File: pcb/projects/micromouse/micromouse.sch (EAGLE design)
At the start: 52 parts, among them M1 332-06, M2 332-06, U1 DSPIC33FJ64MC804-H/PT, U2 UA78M33CKCS, U3 UA78M05CKCS

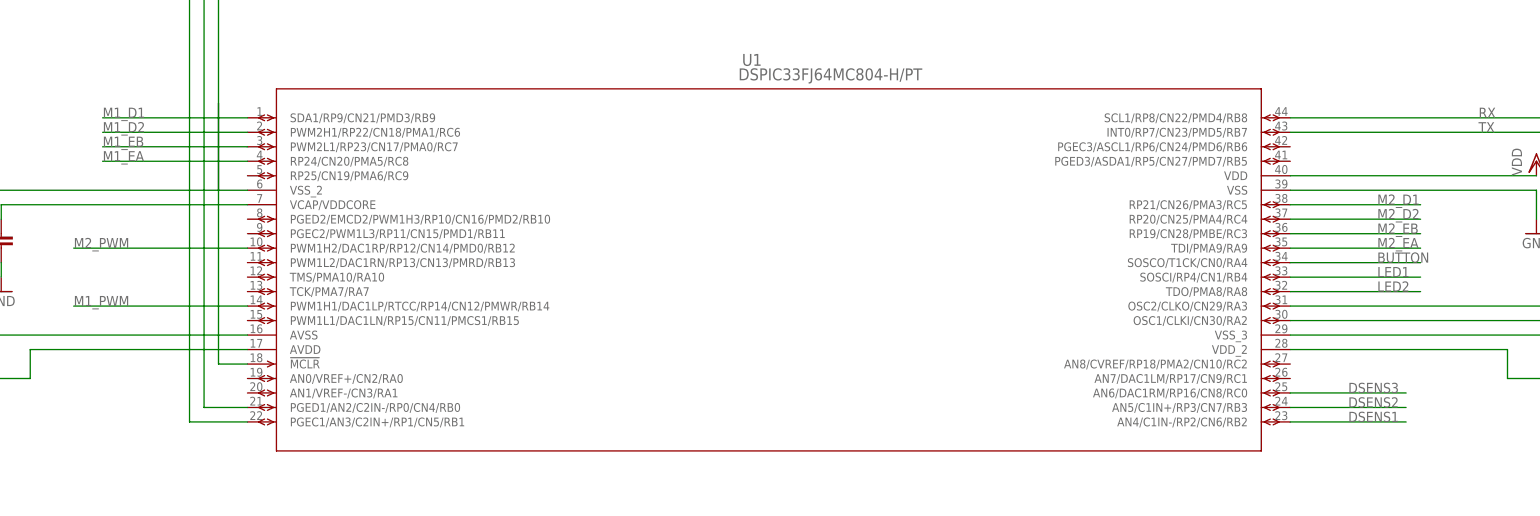
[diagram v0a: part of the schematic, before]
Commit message: Most wiring done
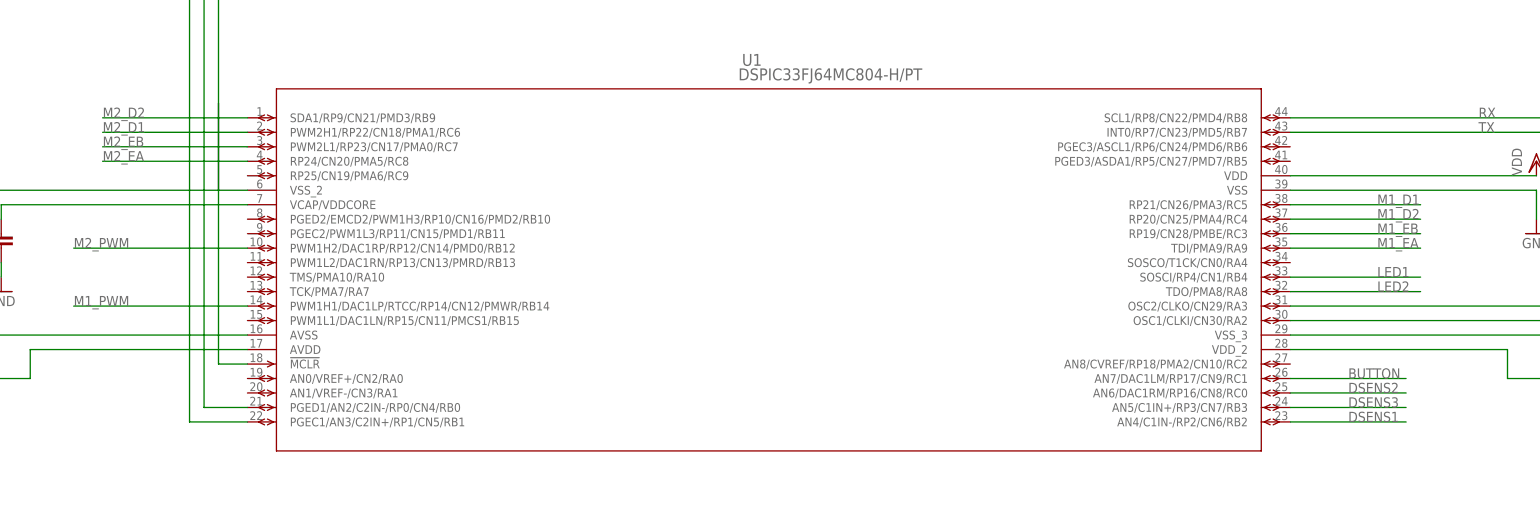
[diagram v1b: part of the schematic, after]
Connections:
- net BUTTON: now also U1.AN7/DAC1LM/RP17/CN9/RC1; no longer U1.SOSCO/T1CK/CN0/RA4
- net DSENS2: now also U1.AN6/DAC1RM/RP16/CN8/RC0; no longer U1.AN5/C1IN+/RP3/CN7/RB3
- net DSENS3: now also U1.AN5/C1IN+/RP3/CN7/RB3; no longer U1.AN6/DAC1RM/RP16/CN8/RC0
- net M1_D1: now also U1.RP21/CN26/PMA3/RC5; no longer U1.SDA1/RP9/CN21/PMD3/RB9
- net M1_D2: now also U1.RP20/CN25/PMA4/RC4; no longer U1.PWM2H1/RP22/CN18/PMA1/RC6
- net M1_EA: now also U1.TDI/PMA9/RA9; no longer U1.RP24/CN20/PMA5/RC8
- net M1_EB: now also U1.RP19/CN28/PMBE/RC3; no longer U1.PWM2L1/RP23/CN17/PMA0/RC7
- net M2_D1: now also U1.PWM2H1/RP22/CN18/PMA1/RC6; no longer U1.RP21/CN26/PMA3/RC5
- net M2_D2: now also U1.SDA1/RP9/CN21/PMD3/RB9; no longer U1.RP20/CN25/PMA4/RC4
- net M2_EA: now also U1.RP24/CN20/PMA5/RC8; no longer U1.TDI/PMA9/RA9
- net M2_EB: now also U1.PWM2L1/RP23/CN17/PMA0/RC7; no longer U1.RP19/CN28/PMBE/RC3
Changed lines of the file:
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@@
 </segment>
 <segment>
-<pinref part="U1" gate="A" pin="PWM2L1/RP23/CN17/PMA0/RC7"/>
-<wire x1="91.44" y1="154.94" x2="116.84" y2="154.94" width="0.1524" layer="91"/>
-<label x="91.44" y="154.94" size="1.778" layer="95"/>
+<pinref part="U1" gate="A" pin="RP19/CN28/PMBE/RC3"/>
+<wire x1="322.58" y1="139.7" x2="299.72" y2="139.7" width="0.1524" layer="91"/>
+<label x="314.96" y="139.7" size="1.778" layer="95"/>
 </segment>
 </net>
@@
 </segment>
 <segment>
-<pinref part="U1" gate="A" pin="RP24/CN20/PMA5/RC8"/>
-<wire x1="91.44" y1="152.4" x2="116.84" y2="152.4" width="0.1524" layer="91"/>
-<label x="91.44" y="152.4" size="1.778" layer="95"/>
+<pinref part="U1" gate="A" pin="TDI/PMA9/RA9"/>
+<wire x1="322.58" y1="137.16" x2="299.72" y2="137.16" width="0.1524" layer="91"/>
+<label x="314.96" y="137.16" size="1.778" layer="95"/>
 </segment>
 </net>
@@
 </segment>
 <segment>
-<pinref part="U1" gate="A" pin="SDA1/RP9/CN21/PMD3/RB9"/>
-<wire x1="91.44" y1="160.02" x2="116.84" y2="160.02" width="0.1524" layer="91"/>
-<label x="91.44" y="160.02" size="1.778" layer="95"/>
+<pinref part="U1" gate="A" pin="RP21/CN26/PMA3/RC5"/>
+<wire x1="322.58" y1="144.78" x2="299.72" y2="144.78" width="0.1524" layer="91"/>
+<label x="314.96" y="144.78" size="1.778" layer="95"/>
 </segment>
 </net>
@@
 </segment>
 <segment>
-<pinref part="U1" gate="A" pin="PWM2H1/RP22/CN18/PMA1/RC6"/>
-<wire x1="91.44" y1="157.48" x2="116.84" y2="157.48" width="0.1524" layer="91"/>
-<label x="91.44" y="157.48" size="1.778" layer="95"/>
+<pinref part="U1" gate="A" pin="RP20/CN25/PMA4/RC4"/>
+<wire x1="322.58" y1="142.24" x2="299.72" y2="142.24" width="0.1524" layer="91"/>
+<label x="314.96" y="142.24" size="1.778" layer="95"/>
 </segment>
 </net>
@@
 </segment>
 <segment>
-<pinref part="U1" gate="A" pin="RP19/CN28/PMBE/RC3"/>
-<wire x1="322.58" y1="139.7" x2="299.72" y2="139.7" width="0.1524" layer="91"/>
-<label x="314.96" y="139.7" size="1.778" layer="95"/>
+<pinref part="U1" gate="A" pin="PWM2L1/RP23/CN17/PMA0/RC7"/>
+<wire x1="91.44" y1="154.94" x2="116.84" y2="154.94" width="0.1524" layer="91"/>
+<label x="91.44" y="154.94" size="1.778" layer="95"/>
 </segment>
 </net>
@@
 </segment>
 <segment>
-<pinref part="U1" gate="A" pin="TDI/PMA9/RA9"/>
-<wire x1="322.58" y1="137.16" x2="299.72" y2="137.16" width="0.1524" layer="91"/>
-<label x="314.96" y="137.16" size="1.778" layer="95"/>
+<pinref part="U1" gate="A" pin="RP24/CN20/PMA5/RC8"/>
+<wire x1="91.44" y1="152.4" x2="116.84" y2="152.4" width="0.1524" layer="91"/>
+<label x="91.44" y="152.4" size="1.778" layer="95"/>
 </segment>
 </net>
@@
 </segment>
 <segment>
-<pinref part="U1" gate="A" pin="RP21/CN26/PMA3/RC5"/>
-<wire x1="322.58" y1="144.78" x2="299.72" y2="144.78" width="0.1524" layer="91"/>
-<label x="314.96" y="144.78" size="1.778" layer="95"/>
+<pinref part="U1" gate="A" pin="PWM2H1/RP22/CN18/PMA1/RC6"/>
+<wire x1="91.44" y1="157.48" x2="116.84" y2="157.48" width="0.1524" layer="91"/>
+<label x="91.44" y="157.48" size="1.778" layer="95"/>
 </segment>
 </net>
@@
 </segment>
 <segment>
-<pinref part="U1" gate="A" pin="RP20/CN25/PMA4/RC4"/>
-<wire x1="322.58" y1="142.24" x2="299.72" y2="142.24" width="0.1524" layer="91"/>
-<label x="314.96" y="142.24" size="1.778" layer="95"/>
+<pinref part="U1" gate="A" pin="SDA1/RP9/CN21/PMD3/RB9"/>
+<wire x1="91.44" y1="160.02" x2="116.84" y2="160.02" width="0.1524" layer="91"/>
+<label x="91.44" y="160.02" size="1.778" layer="95"/>
 </segment>
 </net>
@@
 </segment>
 <segment>
+<pinref part="U1" gate="A" pin="AN6/DAC1RM/RP16/CN8/RC0"/>
+<wire x1="320.04" y1="111.76" x2="299.72" y2="111.76" width="0.1524" layer="91"/>
+<label x="309.88" y="111.76" size="1.778" layer="95"/>
+</segment>
+</net>
+<net name="DSENS3" class="0">
+<segment>
+<wire x1="86.36" y1="195.58" x2="60.96" y2="195.58" width="0.1524" layer="91"/>
+<label x="76.2" y="195.58" size="1.778" layer="95"/>
+<pinref part="DIST3S" gate="1" pin="P"/>
+</segment>
+<segment>
 <pinref part="U1" gate="A" pin="AN5/C1IN+/RP3/CN7/RB3"/>
 <wire x1="320.04" y1="109.22" x2="299.72" y2="109.22" width="0.1524" layer="91"/>
 <label x="309.88" y="109.22" size="1.778" layer="95"/>
-</segment>
-</net>
-<net name="DSENS3" class="0">
-<segment>
-<wire x1="86.36" y1="195.58" x2="60.96" y2="195.58" width="0.1524" layer="91"/>
-<label x="76.2" y="195.58" size="1.778" layer="95"/>
-<pinref part="DIST3S" gate="1" pin="P"/>
-</segment>
-<segment>
-<pinref part="U1" gate="A" pin="AN6/DAC1RM/RP16/CN8/RC0"/>
-<wire x1="320.04" y1="111.76" x2="299.72" y2="111.76" width="0.1524" layer="91"/>
-<label x="309.88" y="111.76" size="1.778" layer="95"/>
 </segment>
 </net>
@@
 </segment>
 <segment>
-<pinref part="U1" gate="A" pin="SOSCO/T1CK/CN0/RA4"/>
-<wire x1="322.58" y1="134.62" x2="299.72" y2="134.62" width="0.1524" layer="91"/>
-<label x="314.96" y="134.62" size="1.778" layer="95"/>
-</segment>
-</net>
+<pinref part="U1" gate="A" pin="AN7/DAC1LM/RP17/CN9/RC1"/>
+<wire x1="320.04" y1="114.3" x2="299.72" y2="114.3" width="0.1524" layer="91"/>
+<label x="309.88" y="114.3" size="1.778" layer="95"/>
+</segment>
+</net>
